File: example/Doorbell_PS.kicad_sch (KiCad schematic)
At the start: 60 parts, among them J1 FROM EXTERNAL 8/16/24VAC CLAS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, J2 7VDC OUTPUT, J3 EXTERNAL LIFEPO4 BATTERY HOLD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, Q101 IRF4905PBF, U1 LM76003RNPT, U2 TPS61088RHLR, U3 LTC4412ES6#TRPBF, U4 AP63205WU-7, U5 BQ25171QWDRCRQ1

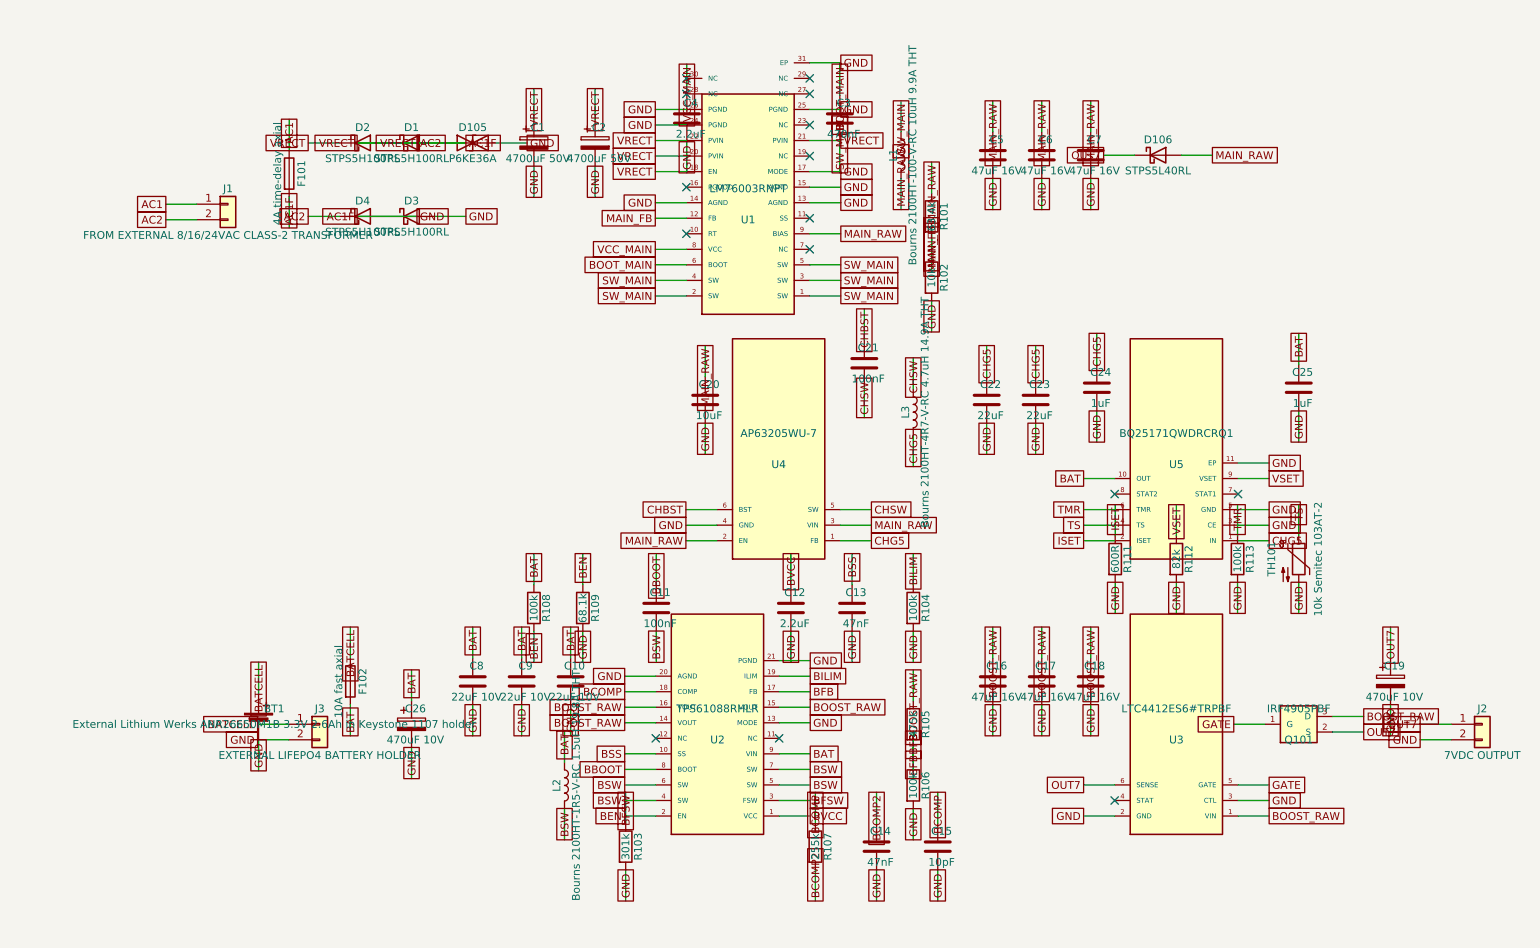
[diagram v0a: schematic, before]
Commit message: klayout v2026.09.17-271-g7e2919c
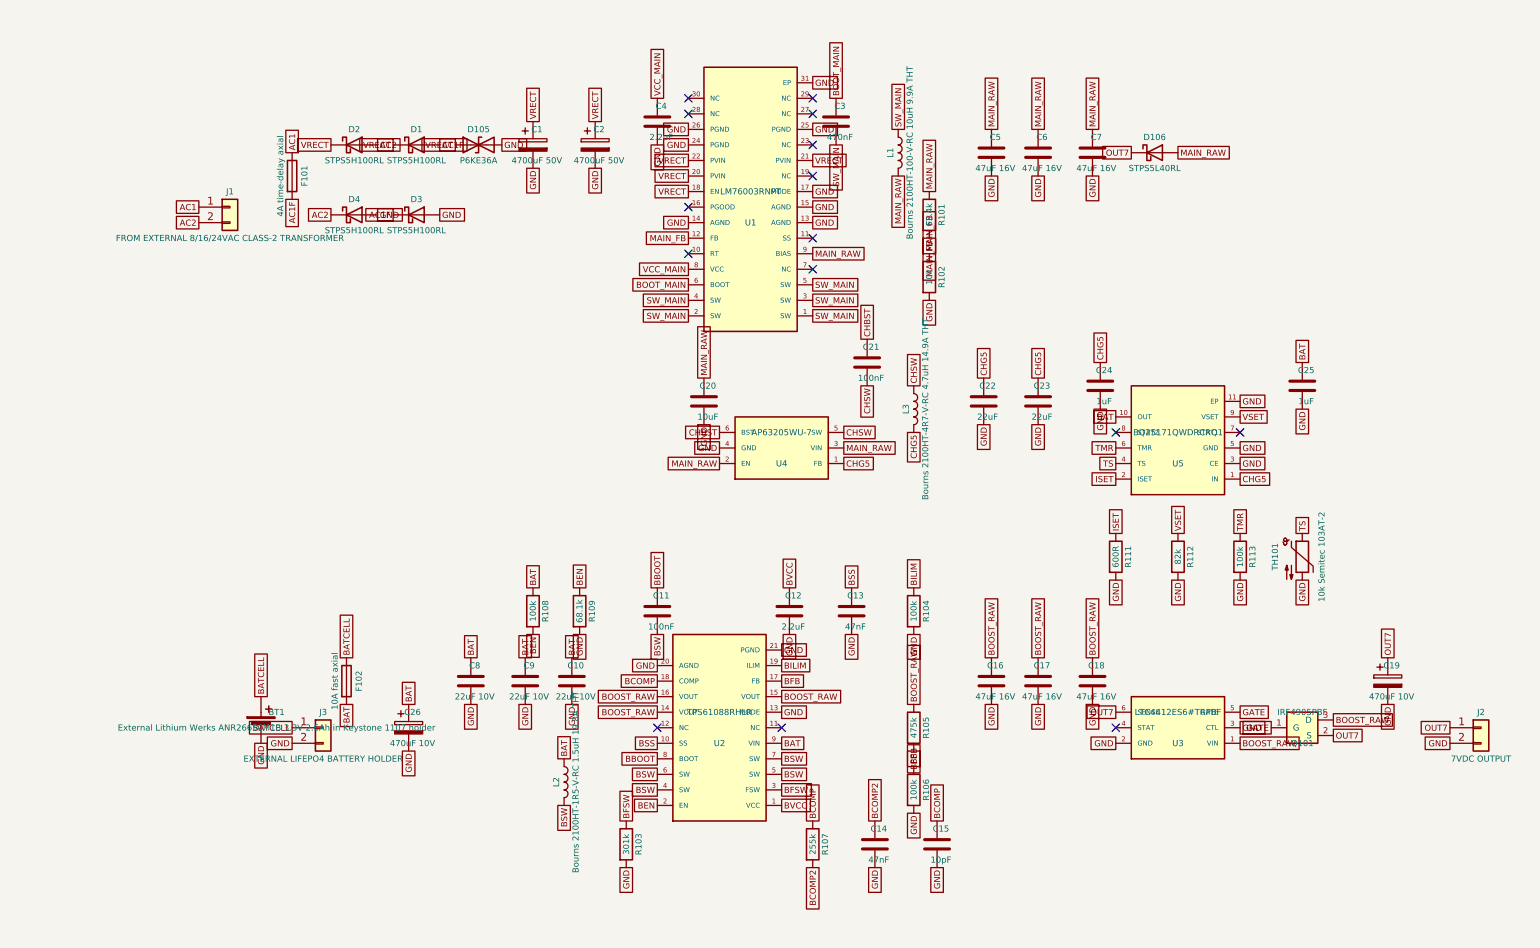
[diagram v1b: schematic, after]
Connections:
- net AC1F: no longer BT1.2 (-), C1.1, C1.2, C10.2, C12.2, C13.2, C14.2, C15.2, C16.2, C17.2, C18.2, C19.2, C2.1, C2.2, C20.2, C22.2, C23.2, C24.2, C25.2, C26.2, C4.2, C5.2, C6.2, C7.2, C8.2, C9.2, D1.1 (K), D105.1 (A1), D105.2 (A2), D2.1 (K), D2.2 (A), D3.2 (A), D4.1 (K), D4.2 (A), J1.2 (Pin_2), J2.2 (Pin_2), J3.2 (Pin_2), R102.2, R103.2, R104.2, R106.2, R109.2, R111.2, R112.2, R113.2, TH101.2, U1.13 (AGND), U1.14 (AGND), U1.15 (AGND), U1.17 (MODE), U1.18 (EN), U1.20 (PVIN), U1.21 (PVIN), U1.22 (PVIN), U1.24 (PGND), U1.25 (PGND), U1.26 (PGND), U1.31 (EP), U2.13 (MODE), U2.20 (AGND), U2.21 (PGND), U3.2 (GND), U3.3 (CTL), U4.4 (GND), U5.11 (EP), U5.3 (CE), U5.5 (GND)
- new net AC2: D2.2 (A), D4.1 (K), J1.2 (Pin_2)
- new net GND: BT1.2 (-), C1.2, C10.2, C12.2, C13.2, C14.2, C15.2, C16.2, C17.2, C18.2, C19.2, C2.2, C20.2, C22.2, C23.2, C24.2, C25.2, C26.2, C4.2, C5.2, C6.2, C7.2, C8.2, C9.2, D105.2 (A2), D3.2 (A), D4.2 (A), J2.2 (Pin_2), J3.2 (Pin_2), R102.2, R103.2, R104.2, R106.2, R109.2, R111.2, R112.2, R113.2, TH101.2, U1.13 (AGND), U1.14 (AGND), U1.15 (AGND), U1.17 (MODE), U1.24 (PGND), U1.25 (PGND), U1.26 (PGND), U1.31 (EP), U2.13 (MODE), U2.20 (AGND), U2.21 (PGND), U3.2 (GND), U3.3 (CTL), U4.4 (GND), U5.11 (EP), U5.3 (CE), U5.5 (GND)
- new net VRECT: C1.1, C2.1, D1.1 (K), D105.1 (A1), D2.1 (K), U1.18 (EN), U1.20 (PVIN), U1.21 (PVIN), U1.22 (PVIN)
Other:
- moved on the sheet: BT1, C11, C12, C13, C17, C22, C24, C25, C26, C3, C4, C6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
